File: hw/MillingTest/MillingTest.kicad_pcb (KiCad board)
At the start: 2 copper layers, 35.6 x 48 mm, 10 parts, among them J1 Conn_ARM_JTAG_SWD_10, U1 CMT2110A, U2 STM32F030F4Px, Y1 Crystal

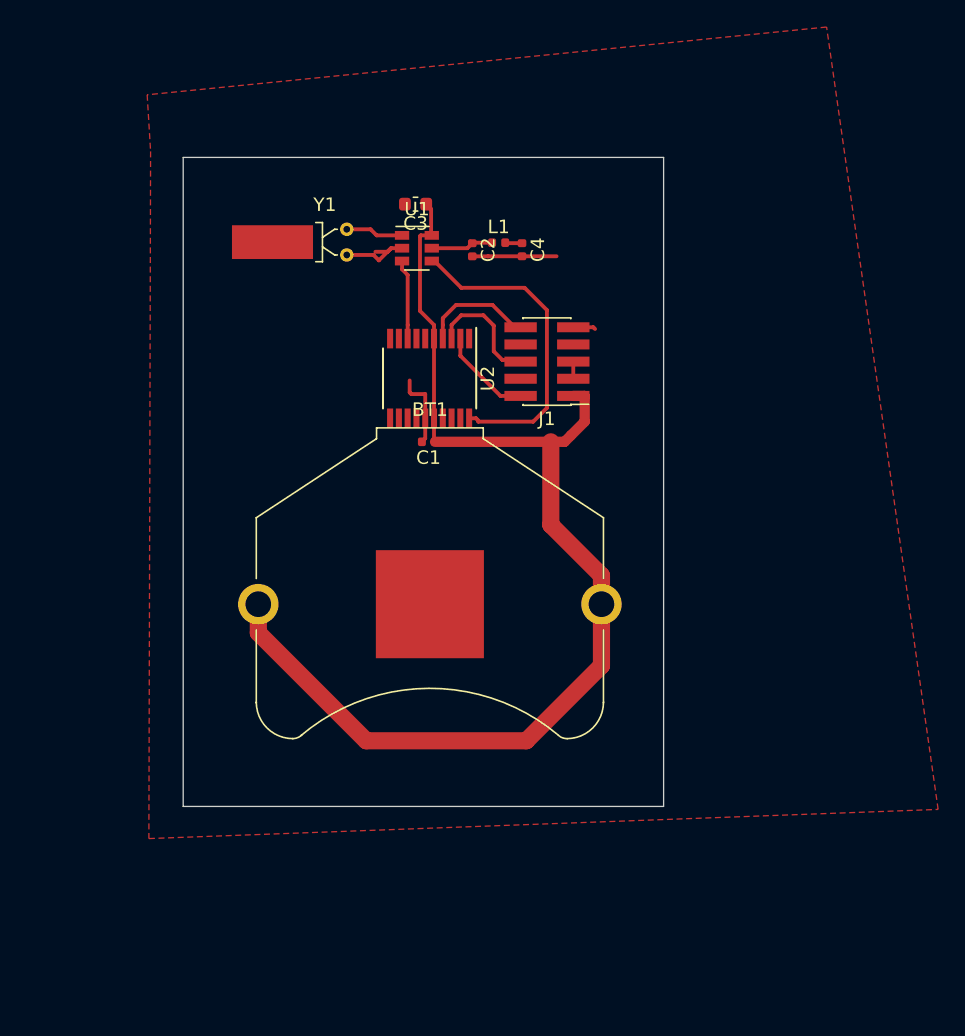
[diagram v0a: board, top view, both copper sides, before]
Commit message: Finished layout with LEDs on board
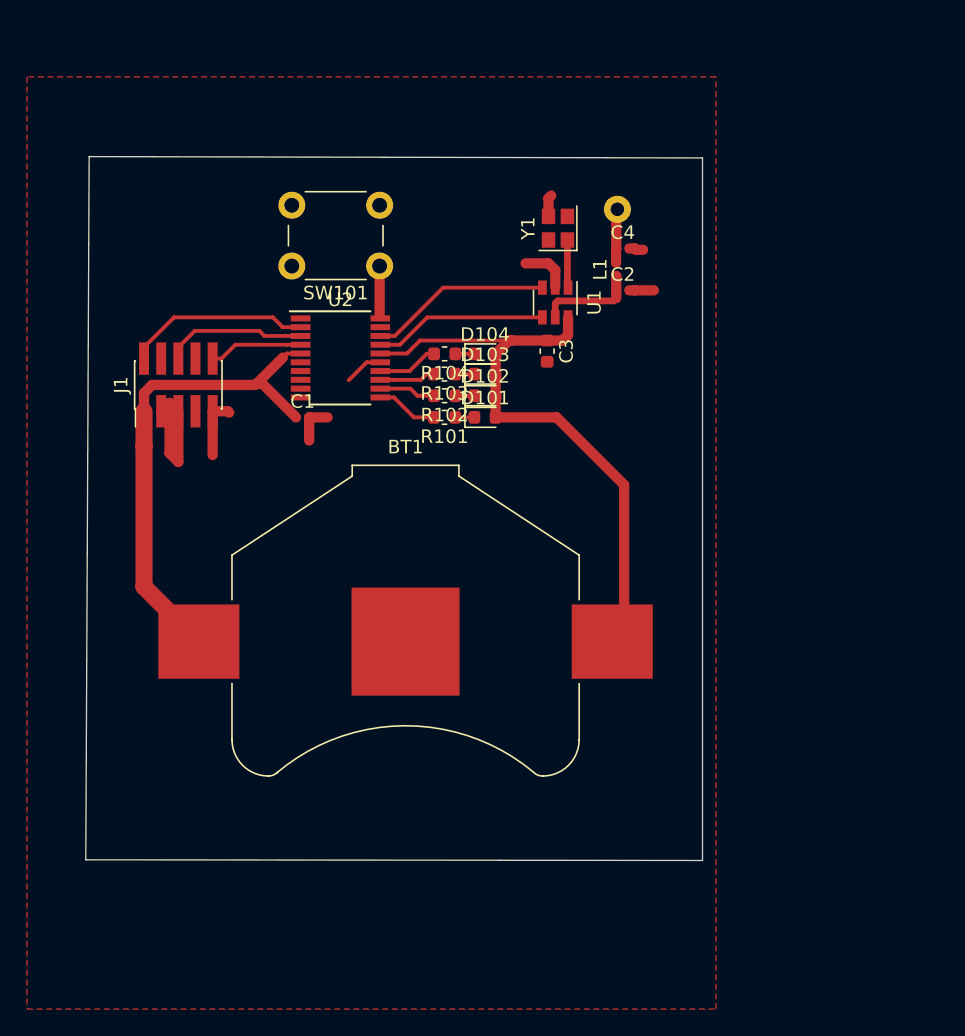
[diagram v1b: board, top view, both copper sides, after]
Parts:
- added AE1: Antenna, TestPoint:TestPoint_THTPad_D2.0mm_Drill1.0mm, B.Cu at (194.7, 64.8)
- added D101: LED, LED_SMD:LED_0603_1608Metric, F.Cu at (184.9, 80.2)
- added D102: LED, LED_SMD:LED_0603_1608Metric, F.Cu at (184.9, 78.6)
- added D103: LED, LED_SMD:LED_0603_1608Metric, F.Cu at (184.9, 77.0)
- added D104: LED, LED_SMD:LED_0603_1608Metric, F.Cu at (184.9, 75.5)
- added R101: R, Resistor_SMD:R_0603_1608Metric, F.Cu at (181.9, 80.2)
- added R102: R, Resistor_SMD:R_0603_1608Metric, F.Cu at (181.9, 78.6)
- added R103: R, Resistor_SMD:R_0603_1608Metric, F.Cu at (181.9, 77.0)
- added R104: R, Resistor_SMD:R_0603_1608Metric, F.Cu at (181.9, 75.5)
- added SW101: SW_Push, Button_Switch_THT:SW_PUSH_6mm, F.Cu at (177.1, 69.0)
- BT1: footprint Battery:BatteryHolder_Keystone_3009_1x2450 -> Battery:BatteryHolder_Keystone_3008_1x2450
- Y1: footprint Crystal:Crystal_DS26_D2.0mm_L6.0mm_Horizontal_1EP_style1 -> Crystal:Crystal_SMD_2520-4Pin_2.5x2.0mm
- moved J1 27.3 mm to (162.2, 77.8), turned to 90 degrees
- moved Y1 15.6 mm to (190.3, 66.2), turned to 90 degrees
- moved C3 14.6 mm to (189.5, 75.3), turned to 270 degrees
- moved C2 11.5 mm to (195.1, 70.8), turned to 0 degrees
- moved U1 11.0 mm to (190.1, 71.7), turned to 270 degrees
- moved C1 9.49 mm to (171.4, 80.2), turned to 0 degrees
- moved L1 8.91 mm to (194.6, 69.2), turned to 90 degrees
- moved C4 7.46 mm to (195.1, 67.7), turned to 0 degrees
- moved U2 6.77 mm to (174.2, 75.8), turned to 0 degrees
- moved BT1 3.30 mm to (179.0, 96.8)
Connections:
- net Net-(BT1-Pad1) renamed /VBAT
- U2 pad 11: (no net) -> Net-(R101-Pad2)
- U2 pad 12: (no net) -> Net-(R102-Pad2)
- U2 pad 13: (no net) -> Net-(R103-Pad2)
- U2 pad 14: (no net) -> Net-(R104-Pad2)
- U2 pad 17: (no net) -> /CLK
- U2 pad 18: (no net) -> /DATA
- U2 pad 20: /CLK -> Net-(SW101-Pad1)
- U2 pad 8: /DATA -> (no net)
- Y1 pad 2: GND -> (no net)
- Y1 pad 3: (no net) -> GND
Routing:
- net /CLK: track 23.6 -> 12.8 mm
- net /DATA: track 5.91 -> 13.5 mm
- net GND: track 20.8 -> 27.9 mm
- net Net-(J1-Pad2): track 6.96 -> 13.6 mm
- net Net-(R101-Pad2): track 0.00 -> 4.57 mm
- net Net-(R104-Pad2): track 0.00 -> 4.53 mm
- net Net-(R102-Pad2): track 0.00 -> 4.19 mm
- net Net-(R103-Pad2): track 0.00 -> 4.14 mm
- net Net-(SW101-Pad1): track 0.00 -> 3.72 mm
- net Net-(AE1-Pad1): track 1.26 -> 4.01 mm
- net Net-(C2-Pad1): track 4.83 -> 7.36 mm
- net Net-(J1-Pad6): track 8.35 -> 10.5 mm
- net Net-(D103-Pad1): track 0.00 -> 1.43 mm
- net Net-(D101-Pad1): track 0.00 -> 1.43 mm
- net Net-(D104-Pad1): track 0.00 -> 1.41 mm
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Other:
- board size 35.6 x 48 mm -> 45.7 x 52.1 mm
